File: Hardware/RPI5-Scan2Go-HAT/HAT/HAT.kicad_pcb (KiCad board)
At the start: 2 copper layers, 85 x 66.5 mm, 34 parts, among them J1 RPi_GPIO, J10 Conn_01x02_Socket, J12 Conn_01x02_Socket, J13 Conn_01x02_Socket, J14 Conn_01x02_Socket, J15 Jack-DC 5V, J18 Conn_01x02_Socket, J19 Conn_01x02_Socket, J2 Conn_01x04_Socket, J20 Conn_01x05_Socket, J21 Conn_01x05_Socket, J22 Conn_01x02_Socket, J23 Conn_01x04_Socket, J24 Conn_01x02_Socket, J3 Conn_01x14_Socket, J4 Conn_01x03_Socket, J5 Conn_01x03_Socket, J6 Conn_01x03_Socket, J7 Conn_01x04_Socket, J8 Conn_01x02_Socket, J9 Conn_01x02_Socket, Q1 DMG2305UX, U1 Pico

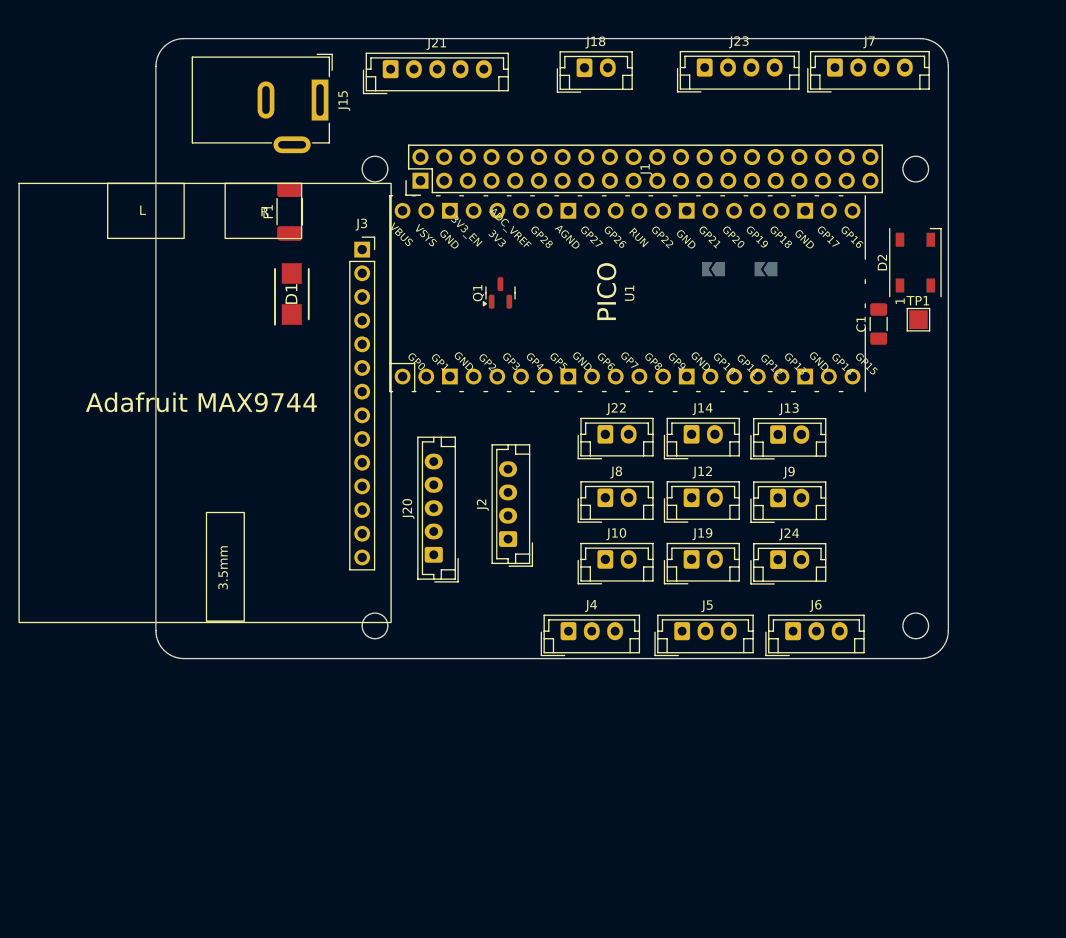
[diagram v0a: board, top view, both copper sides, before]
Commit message: improved layout
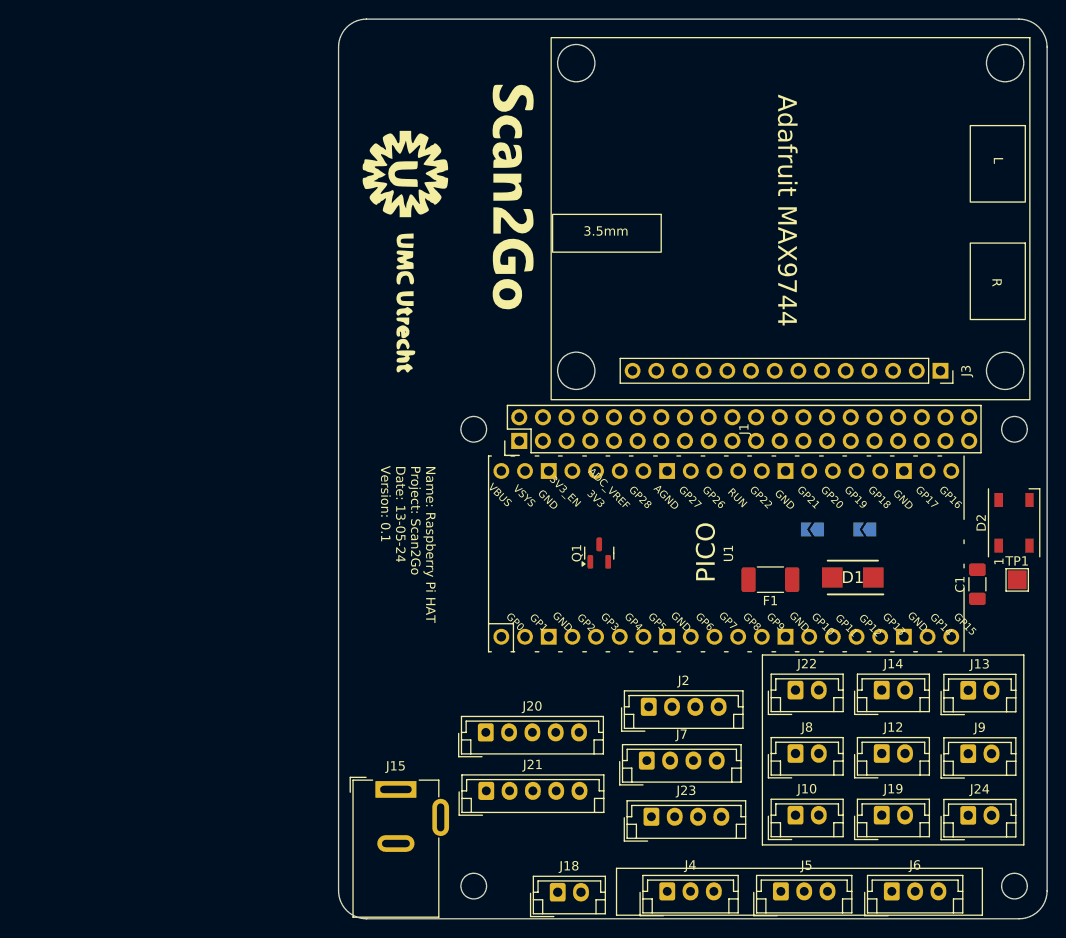
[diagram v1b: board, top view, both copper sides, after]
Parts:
- added G***: LOGO, LOGO, F.Cu at (119.7, 73.9)
- moved J18 88.5 mm to (130.6, 145.6)
- moved J23 80.6 mm to (140.6, 137.5)
- moved J21 78.1 mm to (122.9, 134.7)
- moved J7 77.0 mm to (140.2, 131.4)
- moved J15 74.4 mm to (113.2, 134.5), turned to 0 degrees
- moved D1 67.4 mm to (162.3, 111.8), turned to 180 degrees
- moved F1 64.9 mm to (153.4, 112.0), turned to 180 degrees
- moved J3 63.4 mm to (171.7, 89.6), turned to -90 degrees
- moved J24 34.2 mm to (174.6, 137.3)
- moved J10 34.2 mm to (156.1, 137.3)
- moved J13 34.2 mm to (174.6, 123.9)
- moved J19 34.2 mm to (165.4, 137.3)
- moved J12 34.2 mm to (165.4, 130.7)
- moved J14 34.2 mm to (165.4, 123.9)
- moved J22 34.2 mm to (156.1, 123.9)
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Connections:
- J21 pad 4: Net-(J21-Pin_4) -> (no net)
- U1 pad 36: Net-(J21-Pin_4) -> (no net)
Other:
- board size 85 x 66.5 mm -> 76 x 96.5 mm
- board text added: "Name: Raspberry Pi HAT Project: Scan2Go Date: 13-05-24 Version: 0.1"
